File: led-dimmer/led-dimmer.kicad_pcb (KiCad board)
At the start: 2 copper layers, 33.6 x 33.3 mm, 22 parts, among them J1 Screw_Terminal_01x02, J2 Screw_Terminal_01x02, Q1 IRLML6344, U1 LM555xM

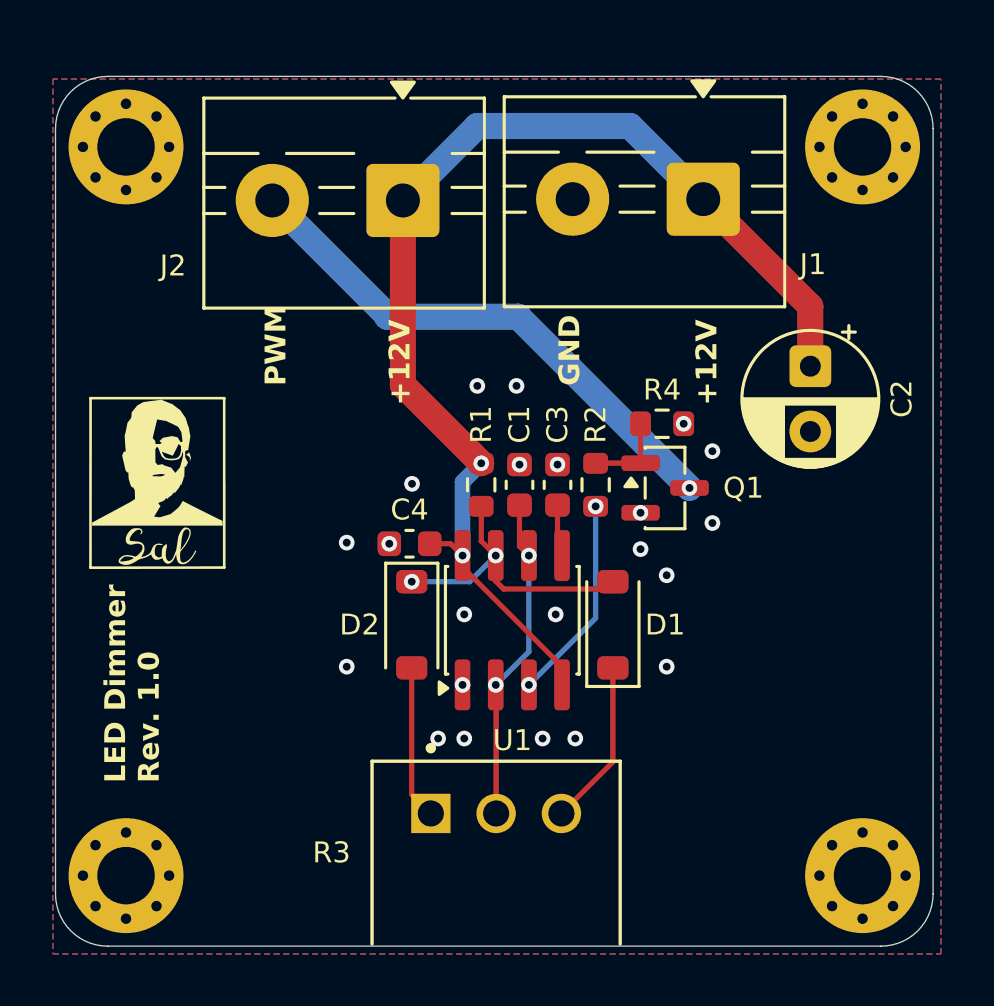
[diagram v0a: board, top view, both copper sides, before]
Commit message: Update LED Dimmer PCB
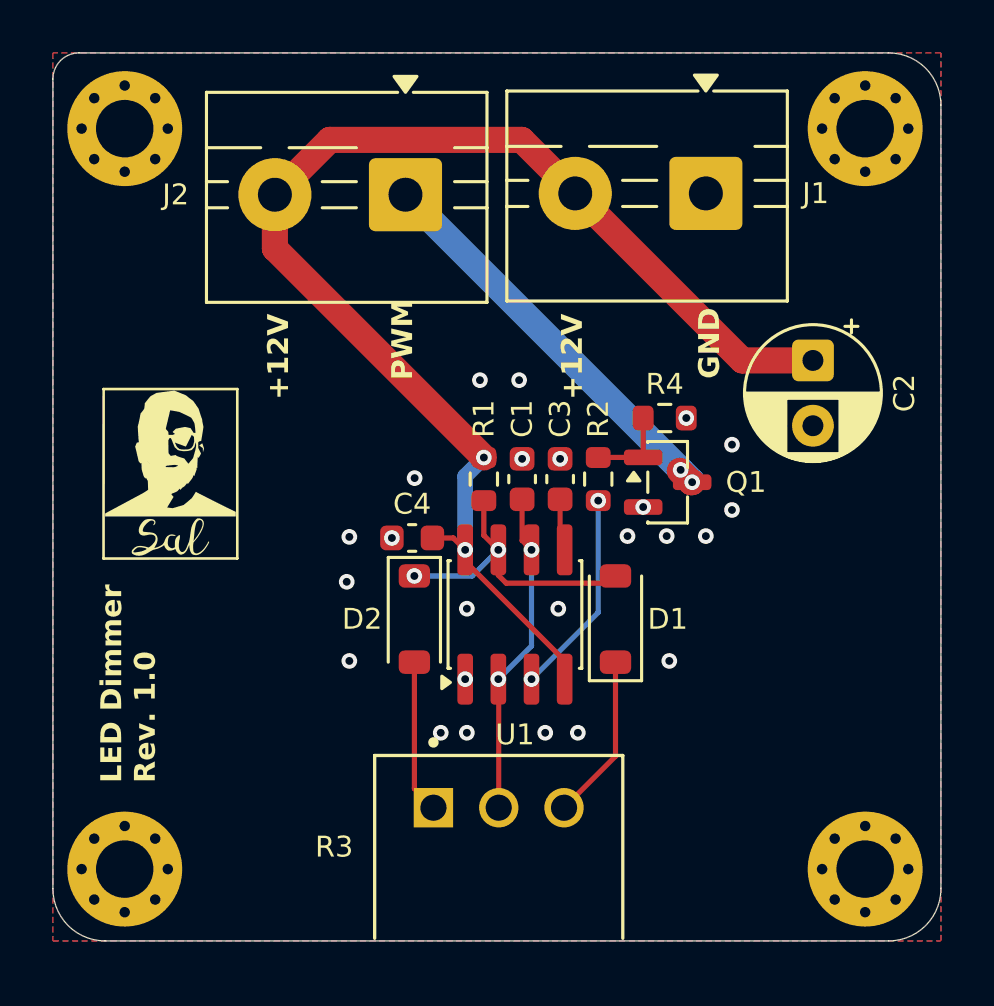
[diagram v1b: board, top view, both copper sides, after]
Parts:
- moved REF** 0.71 mm to (99.1, 98.9)
- moved REF** 0.70 mm to (70.8, 98.9)
- moved G*** 0.61 mm to (72.5, 111.2)
- moved G*** 0.61 mm to (72.5, 114.5)
- moved REF** 0.27 mm to (99.1, 127.2)
- moved REF** 0.25 mm to (70.8, 127.2)
- moved C1 0.24 mm to (86.0, 112.3)
- moved C3 0.24 mm to (87.4, 112.3)
- moved D1 0.24 mm to (89.5, 117.7)
- moved D2 0.24 mm to (81.8, 117.7)
- moved C2 0.24 mm to (97.1, 107.8)
- moved C4 0.24 mm to (81.8, 114.6)
- moved J1 0.24 mm to (93.0, 101.4)
- moved J2 0.24 mm to (81.5, 101.4)
- moved Q1 0.24 mm to (91.5, 112.4)
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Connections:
- J1 pad 1: +12V -> GND
- J1 pad 2: GND -> +12V
- J2 pad 1: +12V -> LED_PWM
- J2 pad 2: LED_PWM -> +12V
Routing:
- net +12V: track 45.2 -> 50.3 mm
- net LED_PWM: track 20.6 -> 16.2 mm, vias 1 -> 2
- net GND: vias 22 -> 24
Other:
- board size 33.6 x 33.3 mm -> 34 x 34 mm
